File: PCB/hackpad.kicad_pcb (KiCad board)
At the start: 2 copper layers, 76.5 x 116.5 mm, 41 parts, among them SW1 SW_Push, SW10 RotaryEncoder_Switch, SW11 SW_Push, SW12 SW_Push, SW13 SW_Push, SW14 SW_Push, SW15 SW_Push, SW16 SW_Push, SW17 SW_Push, SW2 SW_Push, SW3 SW_Push, SW4 SW_Push, SW5 SW_Push, SW6 SW_Push, SW7 SW_Push, SW8 SW_Push, SW9 SW_Push, U1 MOUDLE-SEEEDUINO-XIAO

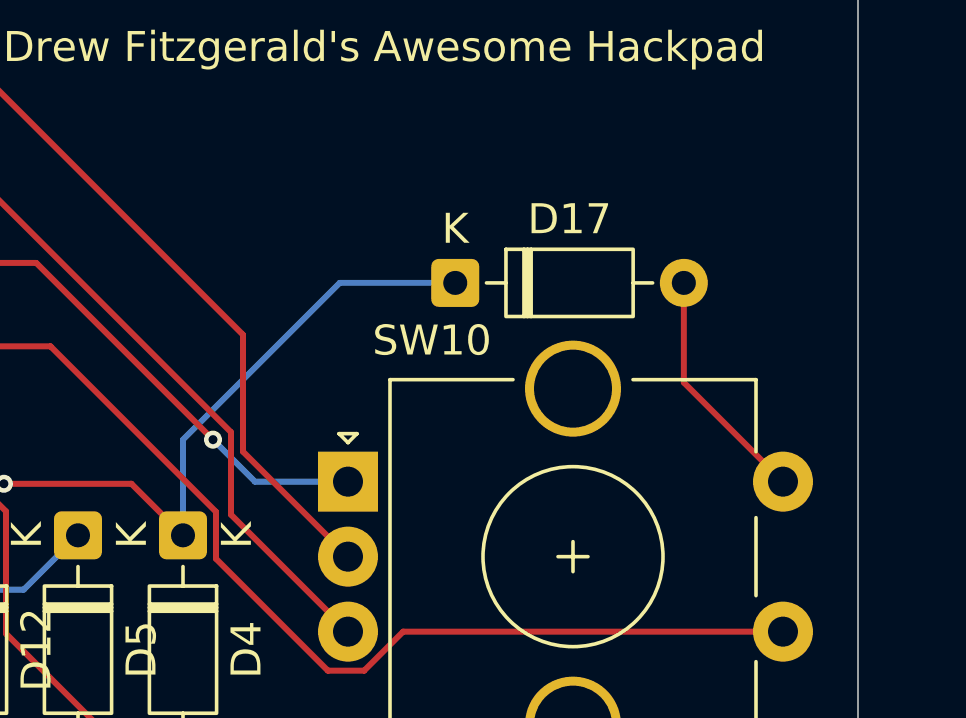
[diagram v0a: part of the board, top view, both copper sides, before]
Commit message: Rah
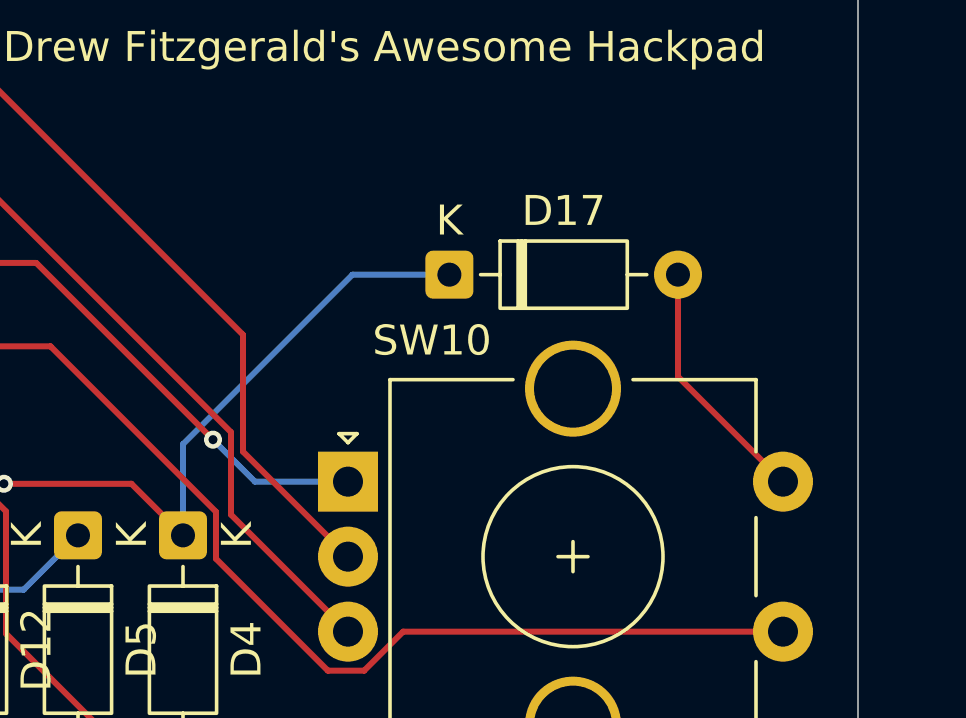
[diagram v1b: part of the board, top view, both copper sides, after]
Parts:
- moved D17 0.34 mm to (151.9, 44.0)
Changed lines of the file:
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@@
 	(footprint "Diode_THT:D_DO-35_SOD27_P7.62mm_Horizontal"
 		(layer "F.Cu")
-		(at 152.075 44.275)
+		(at 151.88 44)
 		(descr "Diode, DO-35_SOD27 series, Axial, Horizontal, pin pitch=7.62mm, length*diameter=4*2mm^2, http://www.diodes.com/_files/packages/DO-35.pdf")
 		(tags "Diode DO-35_SOD27 series Axial Horizontal pin pitch 7.62mm  length 4mm diameter 2mm")
@@
 	)
 	(segment
-		(start 143 49.5)
-		(end 143 52.69)
-		(width 0.2)
-		(layer "B.Cu")
-		(net "ROW1")
-	)
-	(segment
 		(start 137 51)
 		(end 131.6 51)
@@
 	)
 	(segment
-		(start 102.1 53.79)
-		(end 113.9 53.79)
-		(width 0.2)
-		(layer "B.Cu")
-		(net "ROW1")
-	)
-	(segment
-		(start 152.075 44.275)
-		(end 148.225 44.275)
+		(start 148.651471 44)
+		(end 143 49.651471)
 		(width 0.2)
 		(layer "B.Cu")
@@
 	)
 	(segment
-		(start 148.225 44.275)
-		(end 143 49.5)
+		(start 102.1 53.79)
+		(end 113.9 53.79)
 		(width 0.2)
 		(layer "B.Cu")
@@
 	)
 	(segment
+		(start 143 49.651471)
+		(end 143 52.69)
+		(width 0.2)
+		(layer "B.Cu")
+		(net "ROW1")
+	)
+	(segment
 		(start 113.9 53.79)
 		(end 115 52.69)
@@
 	)
 	(segment
+		(start 151.88 44)
+		(end 148.651471 44)
+		(width 0.2)
+		(layer "B.Cu")
+		(net "ROW1")
+	)
+	(segment
 		(start 120.35 66.46)
 		(end 115 61.11)
@@
 	)
 	(segment
-		(start 163 50.9)
-		(end 159.695 47.595)
+		(start 159.5 47.4)
+		(end 159.5 44)
 		(width 0.2)
 		(layer "F.Cu")
@@
 	)
 	(segment
-		(start 159.695 47.595)
-		(end 159.695 44.275)
+		(start 163 50.9)
+		(end 159.5 47.4)
 		(width 0.2)
 		(layer "F.Cu")
